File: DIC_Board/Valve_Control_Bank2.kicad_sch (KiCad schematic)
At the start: 10 parts, among them U21 DRV8823QDCARQ1

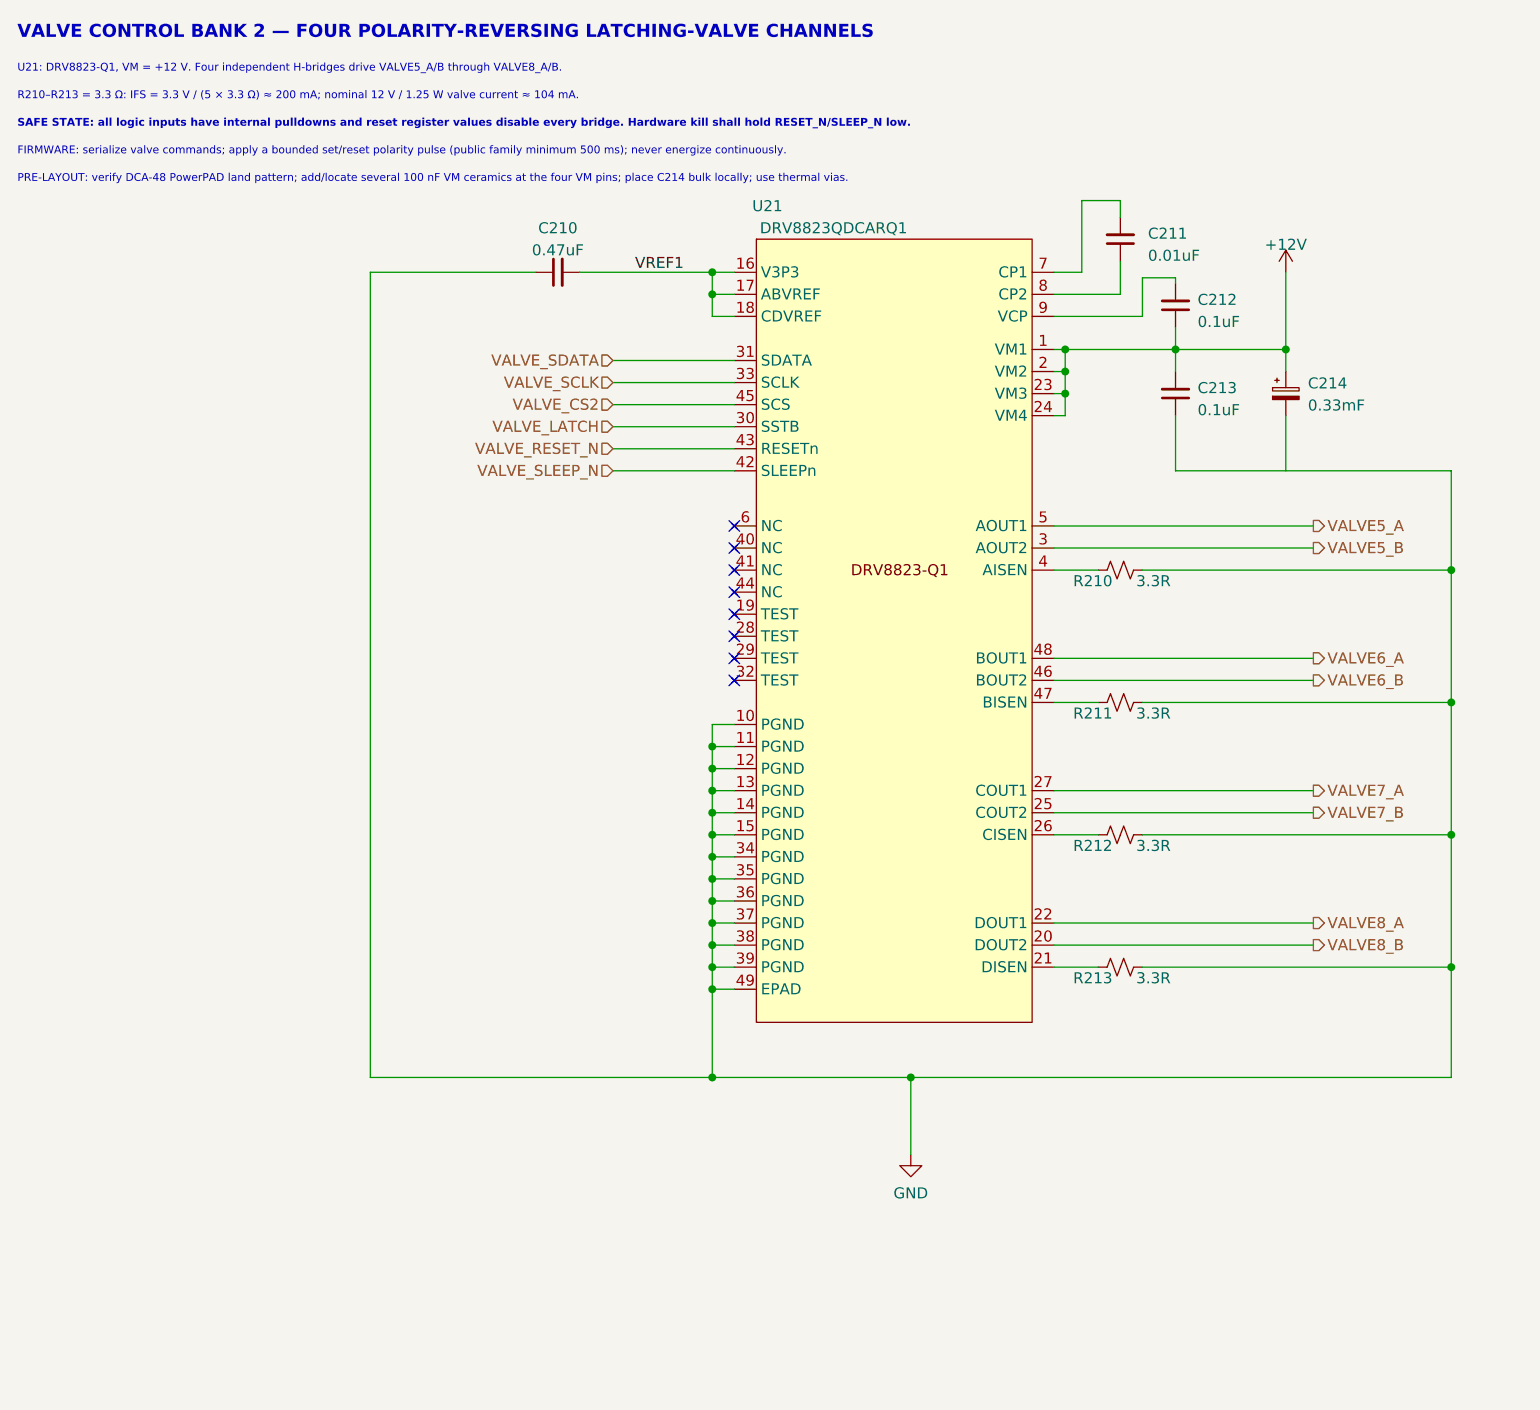
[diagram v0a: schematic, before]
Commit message: Wrapping up schematic
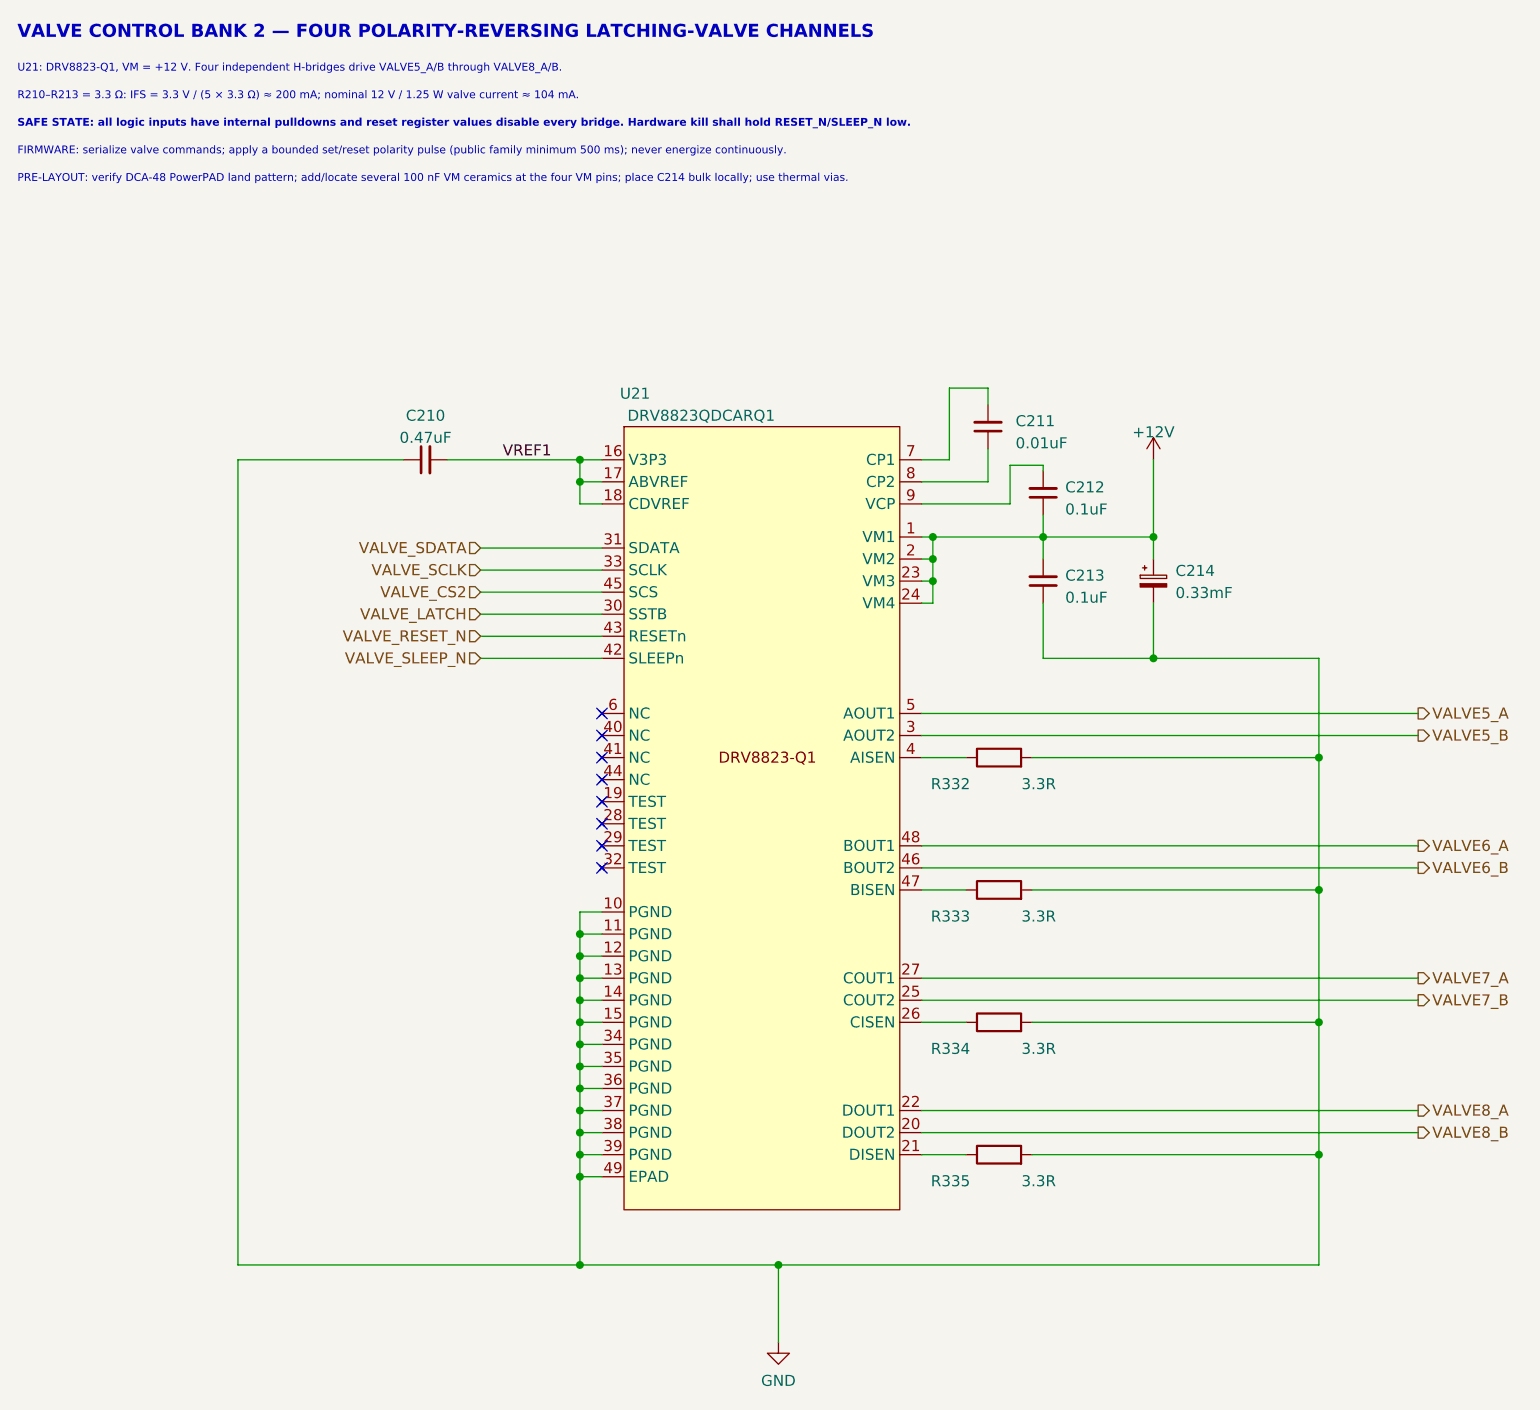
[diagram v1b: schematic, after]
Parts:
- removed R210, R211, R212, R213: 3.3R, Resistor_SMD:R_1206_3216Metric, symbol Device:R_Small_US
- added R332, R333, R334, R335: 3.3R, Resistor_SMD:R_0402_1005Metric, symbol Device:R
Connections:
- net GND: now also C214.2, R332.2, R333.2, R334.2, R335.2
- net at U21.21 (DISEN): now also R335.1
- net at U21.26 (CISEN): now also R334.1
- net at U21.4 (AISEN): now also R332.1
- net at U21.47 (BISEN): now also R333.1
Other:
- moved on the sheet: C210, C211, C212, C213, C214, U21
